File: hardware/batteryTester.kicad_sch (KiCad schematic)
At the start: 43 parts, among them J1 OLED_DISPLAY, J2 USB_C_Receptacle_USB2.0_16P, J3 PROG, Q1 IRF540N, SW1 START, SW2 STOP, SW3 STOP, U1 AMS1117-3.3, U2 LMV321, U3 LMV321, U4 ATSAMD21E15B-A, Y1 32.768kHz

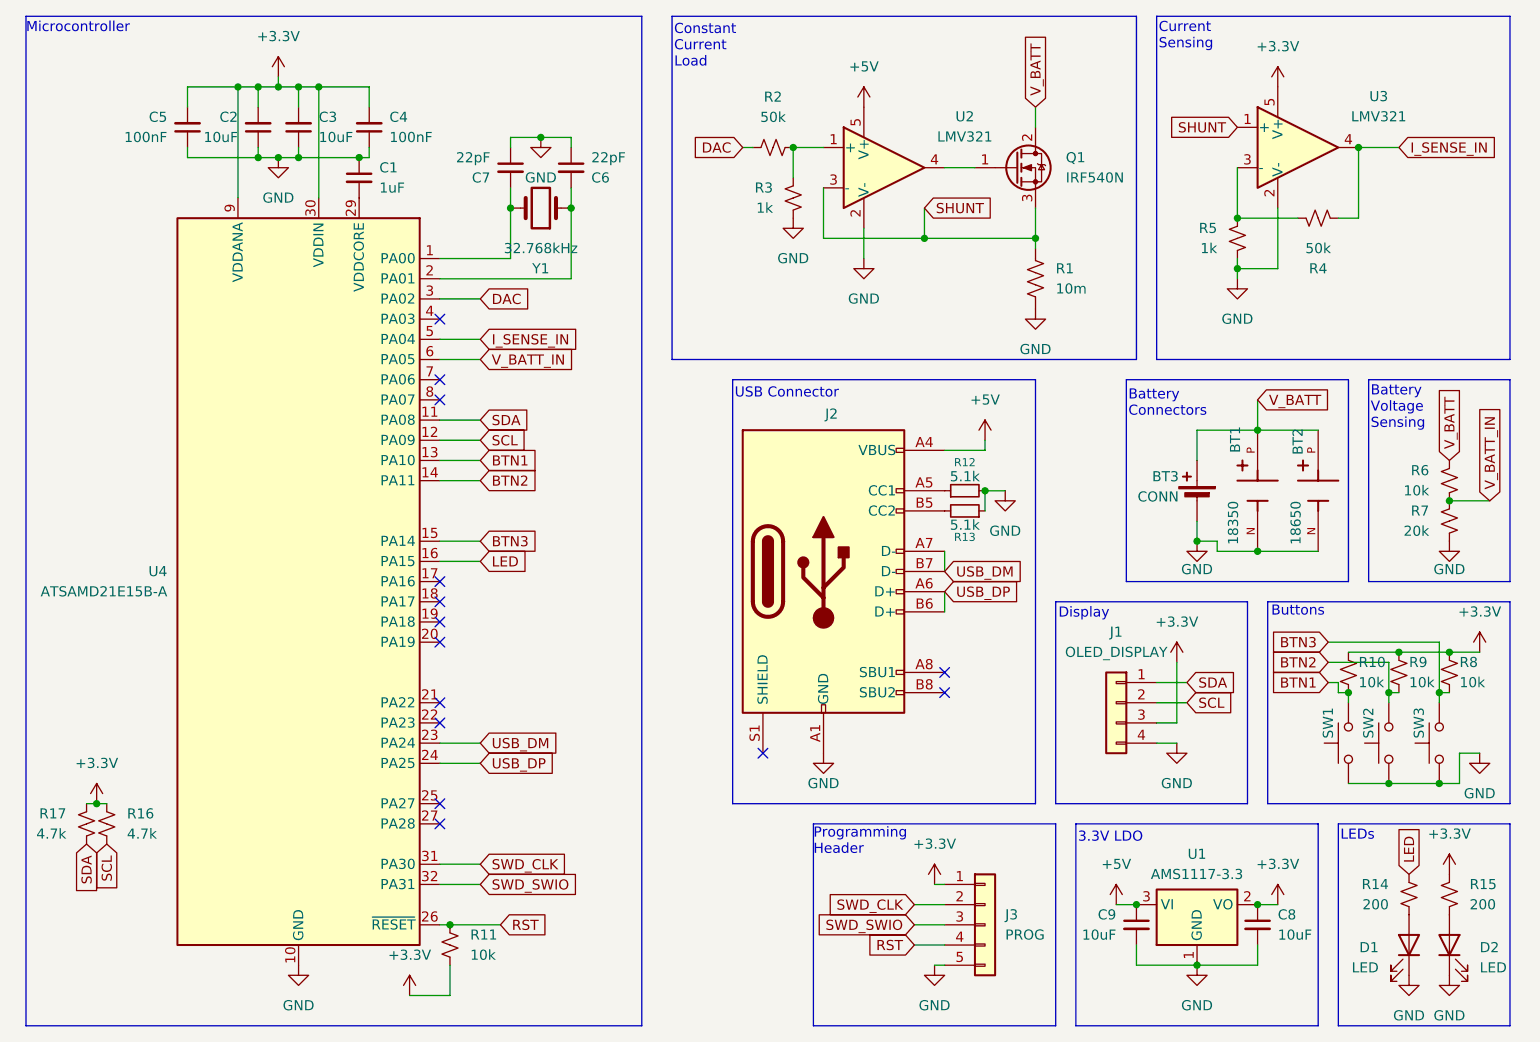
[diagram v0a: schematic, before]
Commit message: re-org for code
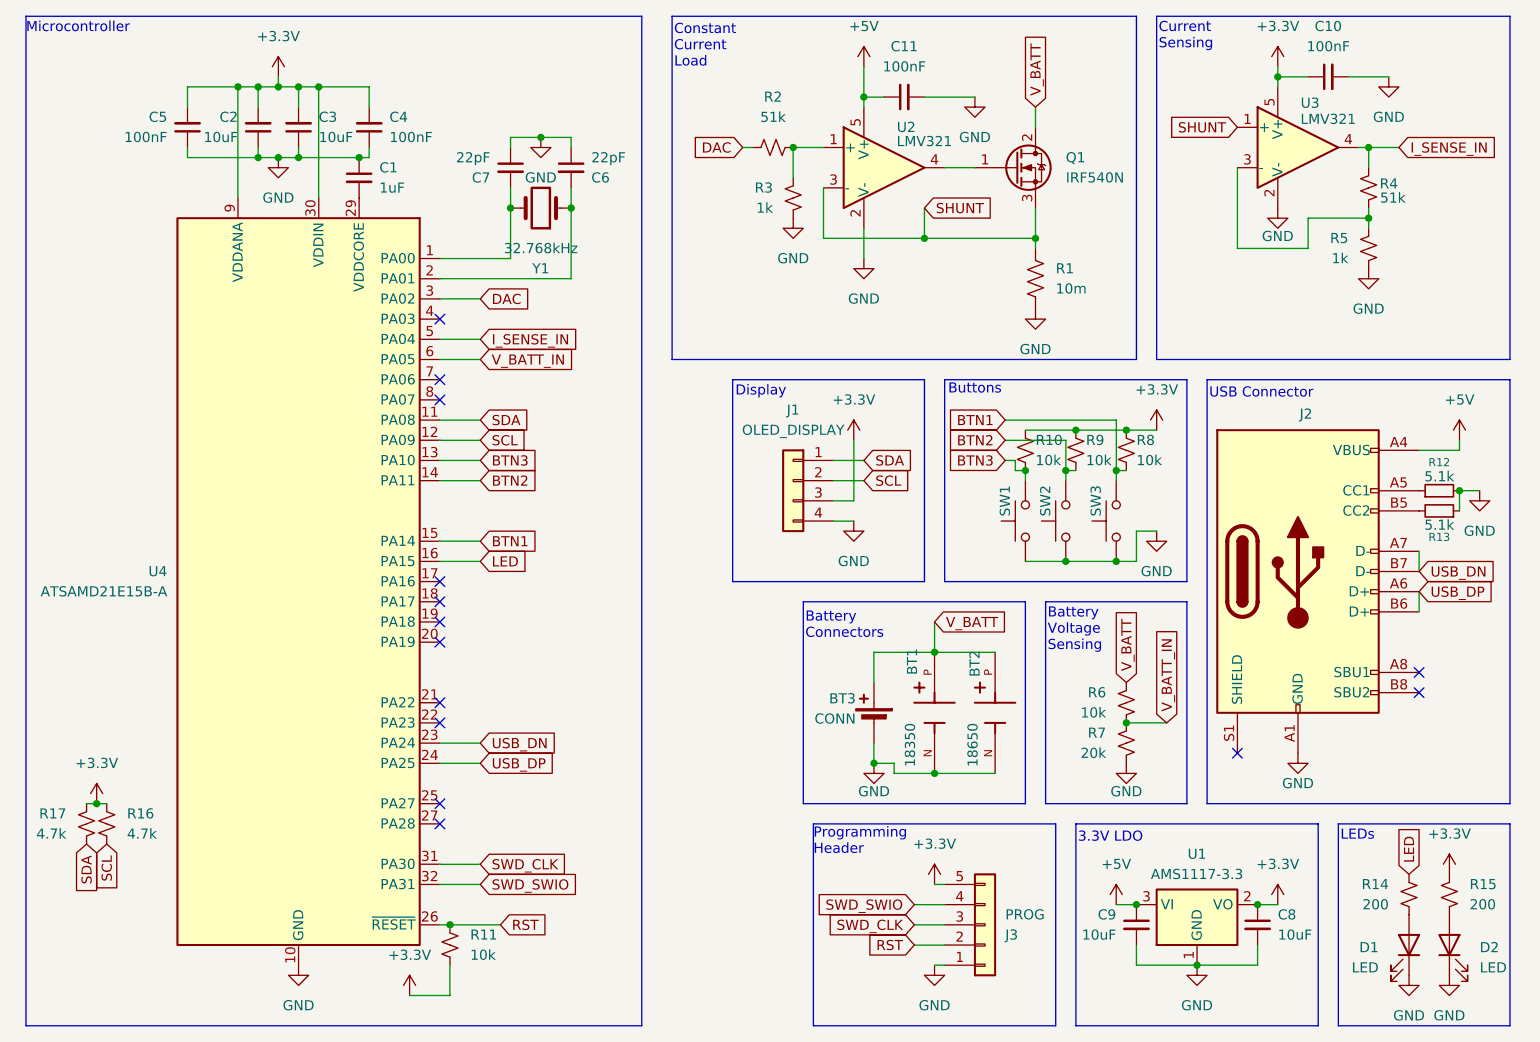
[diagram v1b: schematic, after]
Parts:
- added C10, C11: 100nF, Capacitor_SMD:C_0402_1005Metric, symbol Device:C_Small
- R2, R4: value 50k -> 51k
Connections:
- net +3.3V: now also J3.5 (Pin_5), C10.1; no longer J3.1 (Pin_1)
- net +5V: now also C11.1
- net BTN1: now also R8.2, SW3.2, U4.15 (PA14); no longer R10.2, SW1.2, U4.13 (PA10)
- net BTN3: now also R10.2, SW1.2, U4.13 (PA10); no longer R8.2, SW3.2, U4.15 (PA14)
- net GND: now also J3.1 (Pin_1), C10.2, C11.2; no longer J3.5 (Pin_5)
- net RST: now also J3.2 (Pin_2); no longer J3.4 (Pin_4)
- net SWD_CLK: now also J3.3 (Pin_3); no longer J3.2 (Pin_2)
- net SWD_SWIO: now also J3.4 (Pin_4); no longer J3.3 (Pin_3)
- net USB_DM renamed USB_DN
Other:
- moved on the sheet: BT1, BT2, BT3, J1, J2, R10, R12, R13, R4, R5, R6, R7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
